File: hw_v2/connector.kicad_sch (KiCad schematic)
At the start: 22 parts, among them J1 Conn_02x24_Counter_Clockwise, J14 Conn_01x04, U11 L78M05ABDT-TR, U19 L78M05ABDT-TR, U25 74LVC2G17, U26 74LVC2G17, U8 AMS1117-3.3

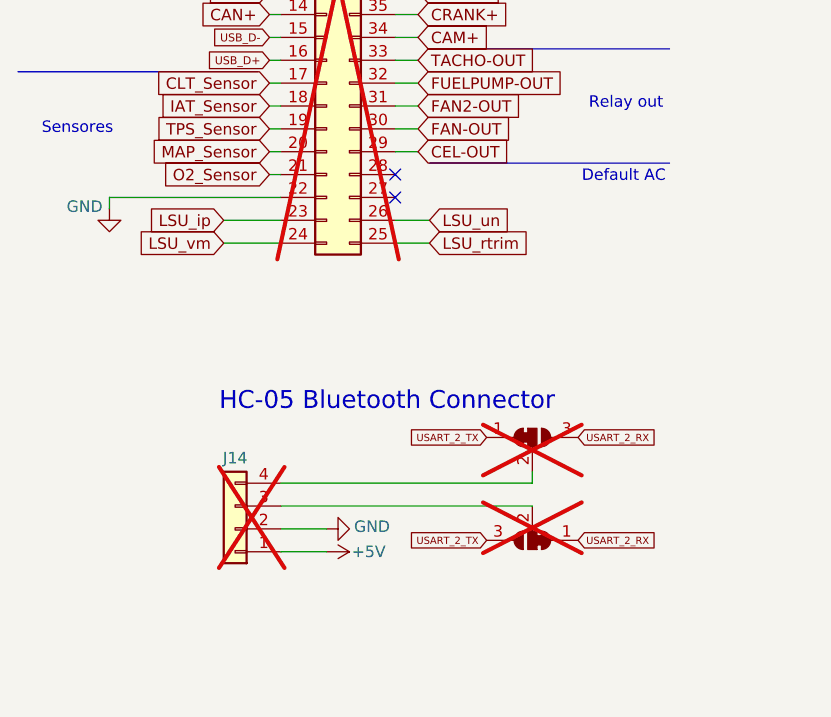
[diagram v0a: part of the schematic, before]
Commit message: wip mcu routing
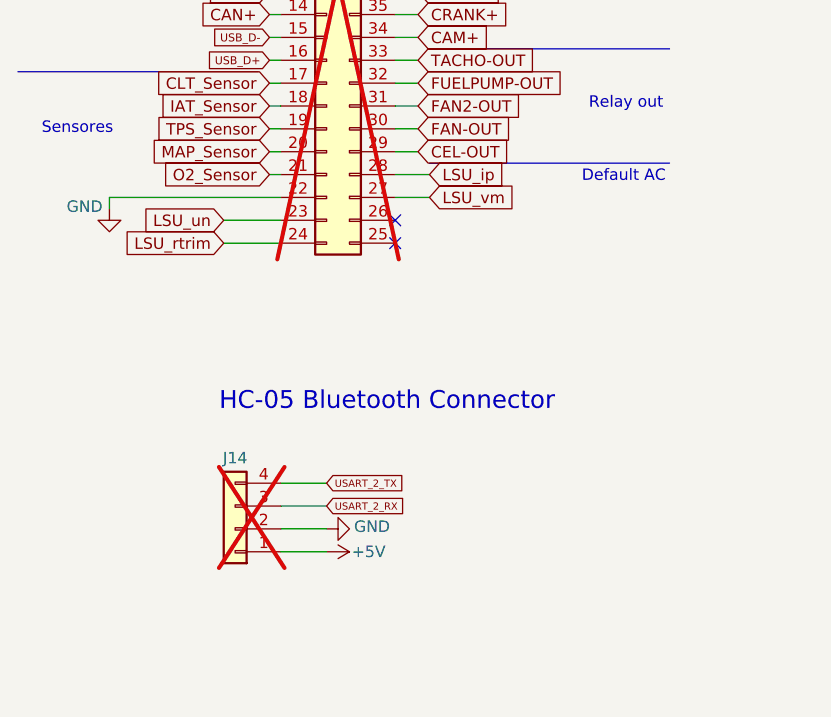
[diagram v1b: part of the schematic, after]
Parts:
- removed JP10, JP9: SolderJumper_3_Bridged12, Jumper:SolderJumper-3_P1.3mm_Bridged2Bar12_Pad1.0x1.5mm, symbol Jumper:SolderJumper_3_Bridged12
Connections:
- net LSU_ip: now also J1.28 (Pin_28); no longer J1.23 (Pin_23)
- net LSU_rtrim: now also J1.24 (Pin_24); no longer J1.25 (Pin_25)
- net LSU_un: now also J1.23 (Pin_23); no longer J1.26 (Pin_26)
- net LSU_vm: now also J1.27 (Pin_27); no longer J1.24 (Pin_24)
- net USART_2_RX: now also J14.3 (Pin_3)
- net USART_2_TX: now also J14.4 (Pin_4)
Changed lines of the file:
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@@
 	)
 	(no_connect
-		(at 86.36 106.68)
+		(at 86.36 111.76)
 	)
 	(no_connect
-		(at 86.36 104.14)
+		(at 86.36 109.22)
 	)
 	(wire
@@
 	(wire
 		(pts
-			(xy 73.66 138.43) (xy 101.6 138.43)
+			(xy 73.66 138.43) (xy 78.74 138.43)
 		)
 		(stroke
@@
 	(wire
 		(pts
-			(xy 101.6 137.16) (xy 101.6 138.43)
-		)
-		(stroke
-			(width 0)
-			(type default)
-		)
-	)
-	(wire
-		(pts
 			(xy 264.16 74.93) (xy 251.46 74.93)
 		)
@@
 	(wire
 		(pts
-			(xy 90.17 109.22) (xy 86.36 109.22)
+			(xy 90.17 104.14) (xy 86.36 104.14)
 		)
 		(stroke
@@
 	(wire
 		(pts
-			(xy 73.66 140.97) (xy 101.6 140.97)
+			(xy 73.66 140.97) (xy 78.74 140.97)
 		)
 		(stroke
@@
 	(wire
 		(pts
-			(xy 90.17 111.76) (xy 86.36 111.76)
+			(xy 90.17 106.68) (xy 86.36 106.68)
 		)
 		(stroke
@@
 	(global_label "USART_2_TX"
 		(shape input)
-		(at 96.52 133.35 180)
+		(at 78.74 138.43 0)
 		(fields_autoplaced yes)
 		(effects
@@
 				(size 0.8 0.8)
 			)
-			(justify right)
+			(justify left)
 		)
 		(property "Intersheetrefs" "${INTERSHEET_REFS}"
-			(at 87.5922 133.35 0)
+			(at 87.6678 138.43 0)
 			(effects
 				(font
 					(size 1.27 1.27)
 				)
-				(justify right)
+				(justify left)
 				(hide yes)
 			)
@@
 	(global_label "LSU_rtrim"
 		(shape input)
-		(at 90.17 111.76 0)
+		(at 67.31 111.76 180)
 		(fields_autoplaced yes)
 		(effects
@@
 				(size 1.27 1.27)
 			)
-			(justify left)
+			(justify right)
 		)
 		(property "Intersheetrefs" "${INTERSHEET_REFS}"
-			(at 102.2871 111.76 0)
+			(at 57.4911 111.76 0)
 			(effects
 				(font
 					(size 1.27 1.27)
 				)
-				(justify left)
+				(justify right)
 				(hide yes)
 			)
@@
 		)
 	)
-	(global_label "USART_2_RX"
-		(shape input)
-		(at 106.68 133.35 0)
-		(fields_autoplaced yes)
-		(effects
-			(font
-				(size 0.8 0.8)
-			)
-			(justify left)
-		)
-		(property "Intersheetrefs" "${INTERSHEET_REFS}"
-			(at 115.7983 133.35 0)
-			(effects
-				(font
-					(size 1.27 1.27)
-				)
-				(justify left)
-				(hide yes)
-			)
-		)
-	)
 	(global_label "IGN-1-OUT"
 		(shape input)
@@
 	(global_label "LSU_un"
 		(shape input)
-		(at 90.17 109.22 0)
+		(at 67.31 109.22 180)
 		(fields_autoplaced yes)
 		(effects
@@
 				(size 1.27 1.27)
 			)
-			(justify left)
+			(justify right)
 		)
 		(property "Intersheetrefs" "${INTERSHEET_REFS}"
-			(at 99.9889 109.22 0)
+			(at 55.1929 109.22 0)
 			(effects
 				(font
 					(size 1.27 1.27)
 				)
-				(justify left)
+				(justify right)
 				(hide yes)
 			)
@@
 		)
 	)
-	(global_label "USART_2_TX"
-		(shape input)
-		(at 96.52 144.78 180)
-		(fields_autoplaced yes)
-		(effects
-			(font
-				(size 0.8 0.8)
-			)
-			(justify right)
-		)
-		(property "Intersheetrefs" "${INTERSHEET_REFS}"
-			(at 87.5922 144.78 0)
-			(effects
-				(font
-					(size 1.27 1.27)
-				)
-				(justify right)
-				(hide yes)
-			)
-		)
-	)
 	(global_label "TPS_Sensor"
 		(shape input)
@@
 	(global_label "USART_2_RX"
 		(shape input)
-		(at 106.68 144.78 0)
+		(at 78.74 140.97 0)
 		(fields_autoplaced yes)
 		(effects
@@
 		)
 		(property "Intersheetrefs" "${INTERSHEET_REFS}"
-			(at 115.7983 144.78 0)
+			(at 87.8583 140.97 0)
 			(effects
 				(font
@@
 	(global_label "LSU_vm"
 		(shape input)
-		(at 67.31 111.76 180)
+		(at 90.17 106.68 0)
 		(fields_autoplaced yes)
 		(effects
@@
 				(size 1.27 1.27)
 			)
-			(justify right)
+			(justify left)
 		)
 		(property "Intersheetrefs" "${INTERSHEET_REFS}"
-			(at 57.1282 111.76 0)
+			(at 99.4447 106.68 0)
 			(effects
 				(font
 					(size 1.27 1.27)
 				)
-				(justify right)
+				(justify left)
 				(hide yes)
 			)
@@
 	(global_label "LSU_ip"
 		(shape input)
-		(at 67.31 109.22 180)
+		(at 90.17 104.14 0)
 		(fields_autoplaced yes)
 		(effects
@@
 				(size 1.27 1.27)
 			)
-			(justify right)
+			(justify left)
 		)
 		(property "Intersheetrefs" "${INTERSHEET_REFS}"
-			(at 58.0353 109.22 0)
+			(at 100.3518 104.14 0)
 			(effects
 				(font
 					(size 1.27 1.27)
 				)
-				(justify right)
+				(justify left)
 				(hide yes)
 			)
@@
 	)
 	(symbol
-		(lib_id "Jumper:SolderJumper_3_Bridged12")
-		(at 101.6 133.35 0)
-		(unit 1)
-		(exclude_from_sim no)
-		(in_bom no)
-		(on_board yes)
-		(dnp yes)
-		(property "Reference" "JP9"
-			(at 101.6 129.54 0)
-			(effects
-				(font
-					(size 1.27 1.27)
-				)
-				(hide yes)
-			)
-		)
-		(property "Value" "SolderJumper_3_Bridged12"
-			(at 101.6 127 0)
-			(effects
-				(font
-					(size 1.27 1.27)
-				)
-				(hide yes)
-			)
-		)
-		(property "Footprint" "Jumper:SolderJumper-3_P1.3mm_Bridged2Bar12_Pad1.0x1.5mm"
-			(at 101.6 133.35 0)
-			(effects
-				(font
-					(size 1.27 1.27)
-				)
-				(hide yes)
-			)
-		)
-		(property "Datasheet" "~"
-			(at 101.6 133.35 0)
-			(effects
-				(font
-					(size 1.27 1.27)
-				)
-				(hide yes)
-			)
-		)
-		(property "Description" "3-pole Solder Jumper, pins 1+2 closed/bridged"
-			(at 101.6 133.35 0)
-			(effects
-				(font
-					(size 1.27 1.27)
-				)
-				(hide yes)
-			)
-		)
-		(pin "3"
-		)
-		(pin "2"
-		)
-		(pin "1"
-		)
-		(instances
-			(project "hw_v1"
-				(path "/b3feb07e-be80-40e1-bd13-6cd54c2f8b0c/312f3a58-86c6-4c57-9da0-ed62046efef3"
-					(reference "JP9")
-					(unit 1)
-				)
-			)
-		)
-	)
-	(symbol
 		(lib_id "Regulator_Linear:AMS1117-3.3")
 		(at 184.15 30.48 0)
@@
 					(unit 1)
 				)
-			)
-		)
-	)
-	(symbol
-		(lib_name "SolderJumper_3_Bridged12_1")
-		(lib_id "Jumper:SolderJumper_3_Bridged12")
-		(at 101.6 144.78 180)
-		(unit 1)
-		(exclude_from_sim no)
-		(in_bom no)
-		(on_board yes)
-		(dnp yes)
-		(fields_autoplaced yes)
-		(property "Reference" "JP10"
-			(at 101.6 148.59 0)
-			(effects
-				(font
-					(size 1.27 1.27)
-				)
-				(hide yes)
-			)
-		)
-		(property "Value" "SolderJumper_3_Bridged12"
-			(at 101.6 151.13 0)
-			(effects
-				(font
-					(size 1.27 1.27)
-				)
-				(hide yes)
-			)
-		)
-		(property "Footprint" "Jumper:SolderJumper-3_P1.3mm_Bridged2Bar12_Pad1.0x1.5mm"
-			(at 101.6 144.78 0)
-			(effects
-				(font
-					(size 1.27 1.27)
-				)
-				(hide yes)
-			)
-		)
-		(property "Datasheet" "~"
-			(at 101.6 144.78 0)
-			(effects
-				(font
-					(size 1.27 1.27)
-				)
-				(hide yes)
-			)
-		)
-		(property "Description" "3-pole Solder Jumper, pins 1+2 closed/bridged"
-			(at 101.6 144.78 0)
-			(effects
-				(font
-					(size 1.27 1.27)
-				)
-				(hide yes)
-			)
-		)
-		(pin "3"
-		)
-		(pin "2"
-		)
-		(pin "1"
-		)
-		(instances
-			(project "hw_v1"
-				(path "/b3feb07e-be80-40e1-bd13-6cd54c2f8b0c/312f3a58-86c6-4c57-9da0-ed62046efef3"
-					(reference "JP10")
-					(unit 1)
-				)
